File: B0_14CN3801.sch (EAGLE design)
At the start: 23 parts

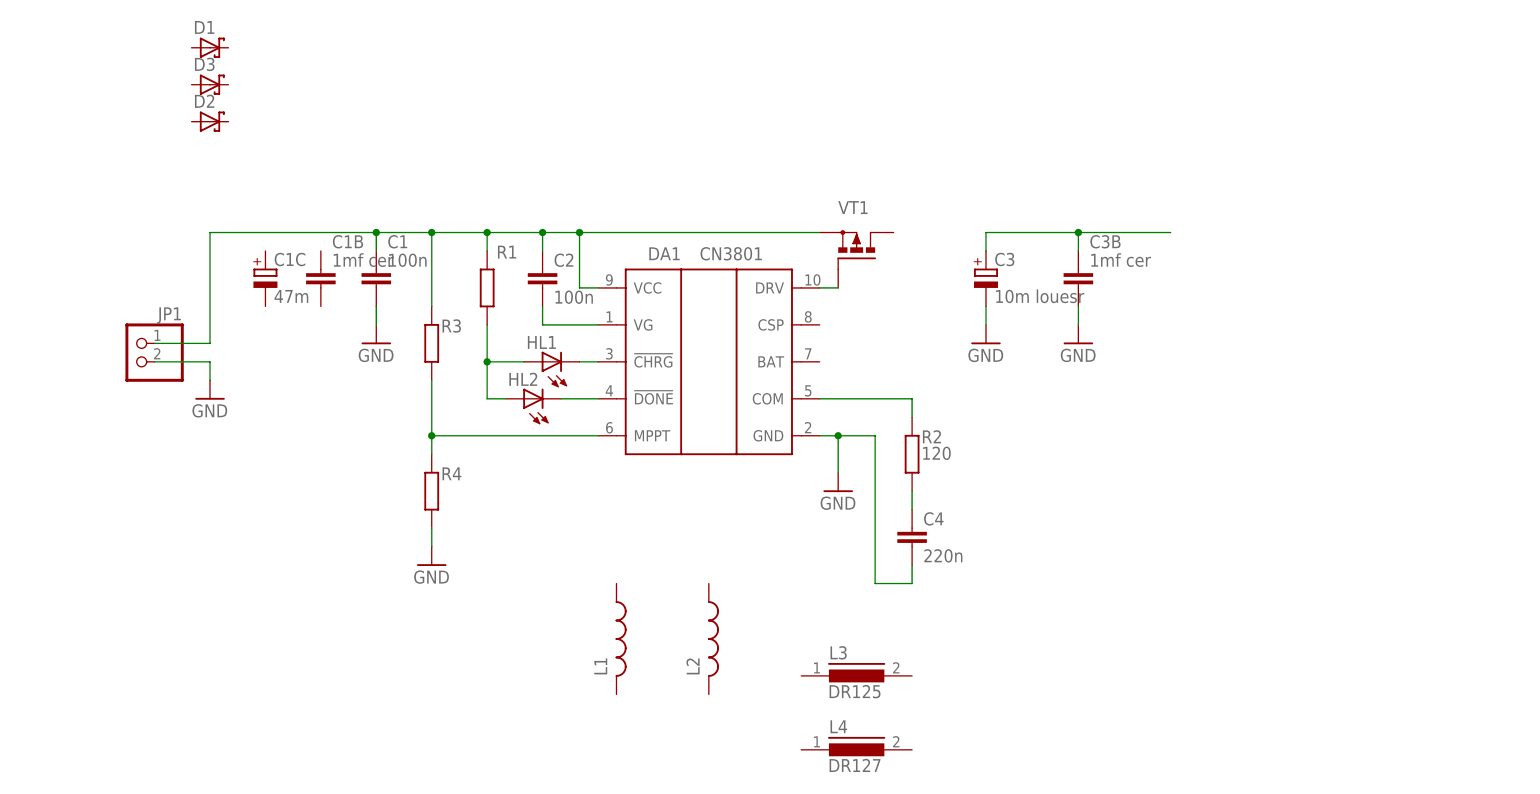
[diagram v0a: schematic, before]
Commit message: .
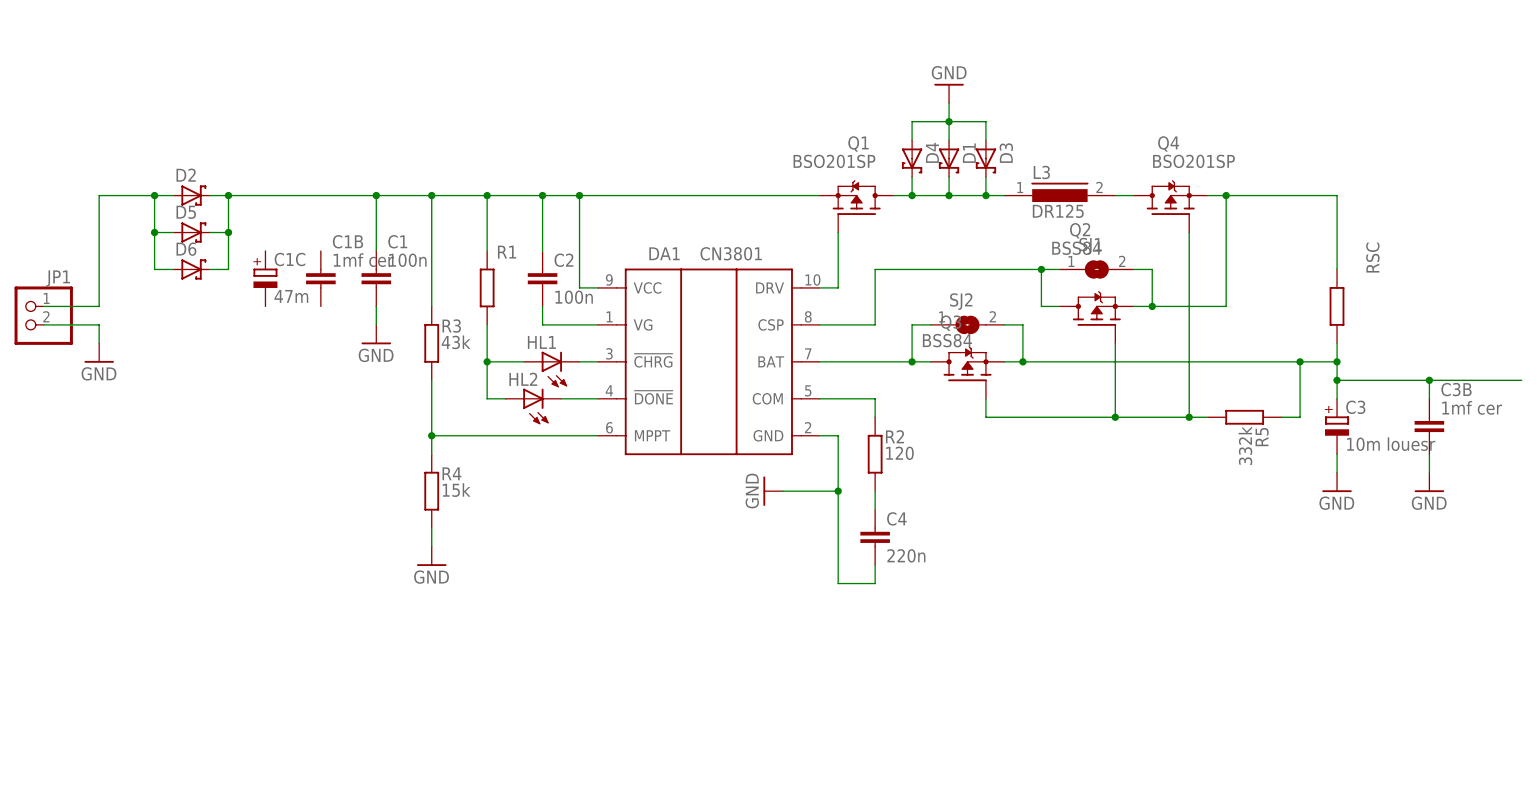
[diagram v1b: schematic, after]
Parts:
- removed L1: (no value), rcl:L-USPIS2816
- removed L2: (no value), rcl:L-USWE-TPC
- removed L4: DR127, inductors:DR127
- removed VT1: (no value), m_transistor:MOSFET-P_TO220_V
- added D4, D5, D6: (no value), diode:SCHOTTKY-DIODESMC
- added Q1, Q4: BSO201SP, transistor-fet:BSO201SP
- added Q2, Q3: BSS84, transistor-fet:BSA223SP
- added R5: 332k, rcl:R-EU_R0805
- added RSC: (no value), rcl:R-EU_R0805
- added SJ1, SJ2: (no value), jumper:SJ
- R3: value (none) -> 43k
- R4: value (none) -> 15k
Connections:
- removed net N$10: C3.+, C3B.1
- new net BAT: DA1.BAT, Q3.D, SJ2.1
- new net CSP: DA1.CSP, Q2.D, SJ1.1
- new net N$11: L3.2, Q4.D
- new net N$12: Q2.G, Q3.G, Q4.G, R5.1
- new net N$13: D1.C, D3.C, D4.C, L3.1, Q1.D
- new net N$14: Q2.S, Q4.S, RSC.2, SJ1.2
- new net N$15: C3.+, C3B.1, Q3.S, R5.2, RSC.1, SJ2.2
- new net N$4: D2.A, D5.A, D6.A, JP1.1
- net GND: now also D1.A, D3.A, D4.A
- net N$1: now also D2.C, D5.C, D6.C, Q1.S; no longer JP1.1, VT1.S
- net N$9: now also Q1.G; no longer VT1.G
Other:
- moved on the sheet: C3, C3B, C4, D1, D2, D3, JP1, L3, R2
